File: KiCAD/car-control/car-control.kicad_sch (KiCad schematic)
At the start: 25 parts, among them J1 USB_B_Micro, J2 Conn_01x06, J3 USB_A, J4 Conn_01x04, SW1 SW_Push, SW2 SW_Push, SW3 SW_Push, SW4 SW_Push, SW5 COM-15140, U1 OLED-SSD1322

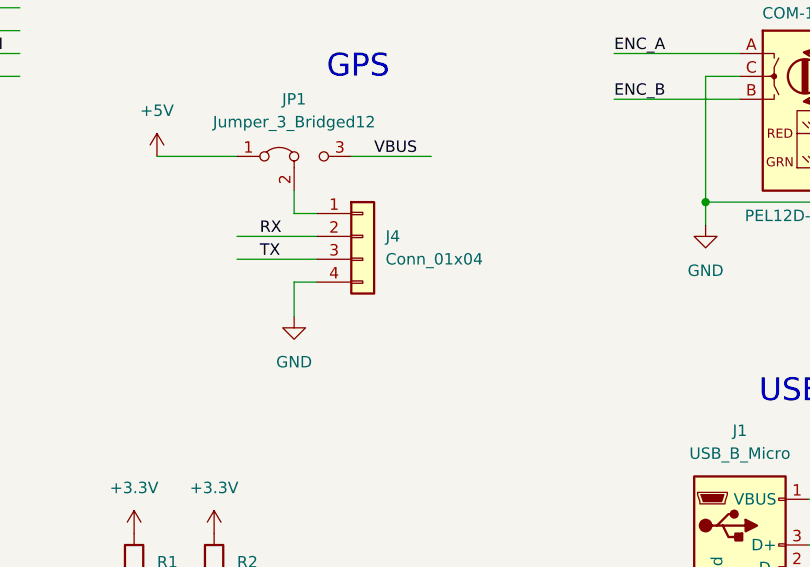
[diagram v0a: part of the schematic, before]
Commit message: PCB V1.0 as built
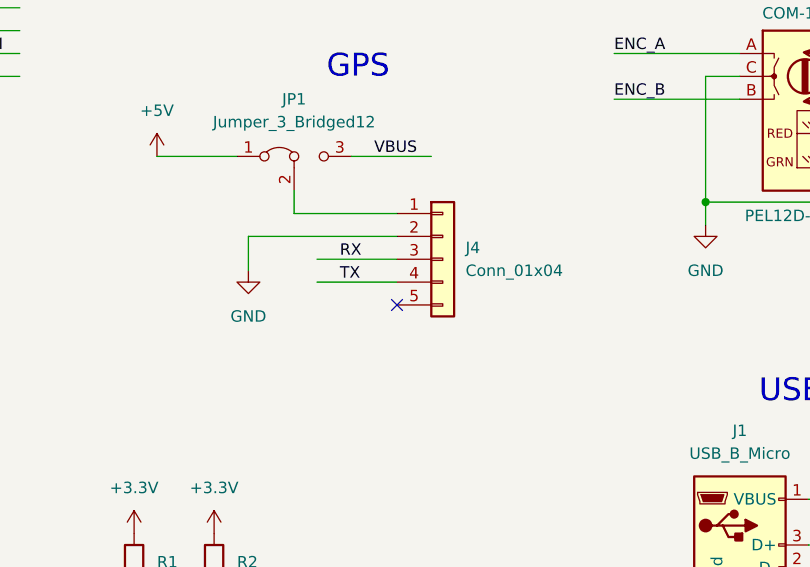
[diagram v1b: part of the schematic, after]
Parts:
- J4: footprint Connector_PinSocket_2.54mm:PinSocket_1x04_P2.54mm_Vertical -> Connector_PinSocket_2.54mm:PinSocket_1x05_P2.54mm_Vertical; symbol Connector_Generic:Conn_01x04 -> Connector_Generic:Conn_01x05
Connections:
- net GND: now also J4.2 (Pin_2); no longer J4.4 (Pin_4)
- net RX: now also J4.3 (Pin_3); no longer J4.2 (Pin_2)
- net TX: now also J4.4 (Pin_4); no longer J4.3 (Pin_3)
- no-connect marks 2 -> 3
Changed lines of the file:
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@@
+	)
+	(no_connect
+		(at 134.62 116.84)
 	)
 	(no_connect
@@
 	(wire
 		(pts
-			(xy 116.84 109.22) (xy 125.73 109.22)
+			(xy 125.73 111.76) (xy 134.62 111.76)
 		)
 		(stroke
@@
 	(wire
 		(pts
-			(xy 125.73 106.68) (xy 123.19 106.68)
+			(xy 123.19 106.68) (xy 134.62 106.68)
 		)
 		(stroke
@@
 	(wire
 		(pts
-			(xy 116.84 111.76) (xy 125.73 111.76)
+			(xy 125.73 114.3) (xy 134.62 114.3)
 		)
 		(stroke
@@
 	(wire
 		(pts
-			(xy 123.19 114.3) (xy 123.19 118.11)
+			(xy 118.11 109.22) (xy 118.11 113.03)
 		)
 		(stroke
@@
 	(wire
 		(pts
-			(xy 125.73 114.3) (xy 123.19 114.3)
+			(xy 118.11 109.22) (xy 134.62 109.22)
 		)
 		(stroke
@@
 	)
 	(label "RX"
-		(at 119.38 109.22 0)
+		(at 128.27 111.76 0)
 		(effects
 			(font
@@
 	)
 	(label "TX"
-		(at 119.38 111.76 0)
+		(at 128.27 114.3 0)
 		(effects
 			(font
@@
 	(symbol
 		(lib_id "power:GND")
-		(at 123.19 118.11 0)
+		(at 118.11 113.03 0)
 		(unit 1)
 		(exclude_from_sim no)
@@
 		(fields_autoplaced yes)
 		(property "Reference" "#PWR014"
-			(at 123.19 124.46 0)
+			(at 118.11 119.38 0)
 			(effects
 				(font
@@
 		)
 		(property "Value" "GND"
-			(at 123.19 123.19 0)
+			(at 118.11 118.11 0)
 			(effects
 				(font
@@
 		)
 		(property "Footprint" ""
-			(at 123.19 118.11 0)
+			(at 118.11 113.03 0)
 			(effects
 				(font
@@
 		)
 		(property "Datasheet" ""
-			(at 123.19 118.11 0)
+			(at 118.11 113.03 0)
 			(effects
 				(font
@@
 		)
 		(property "Description" ""
-			(at 123.19 118.11 0)
+			(at 118.11 113.03 0)
 			(effects
 				(font
@@
 	)
 	(symbol
-		(lib_id "Connector_Generic:Conn_01x04")
-		(at 130.81 109.22 0)
+		(lib_id "Connector_Generic:Conn_01x05")
+		(at 139.7 111.76 0)
 		(unit 1)
 		(exclude_from_sim no)
@@
 		(fields_autoplaced yes)
 		(property "Reference" "J4"
-			(at 133.35 109.2199 0)
+			(at 142.24 110.4899 0)
 			(effects
 				(font
@@
 		)
 		(property "Value" "Conn_01x04"
-			(at 133.35 111.7599 0)
+			(at 142.24 113.0299 0)
 			(effects
 				(font
@@
 			)
 		)
-		(property "Footprint" "Connector_PinSocket_2.54mm:PinSocket_1x04_P2.54mm_Vertical"
-			(at 130.81 109.22 0)
+		(property "Footprint" "Connector_PinSocket_2.54mm:PinSocket_1x05_P2.54mm_Vertical"
+			(at 139.7 111.76 0)
 			(effects
 				(font
@@
 		)
 		(property "Datasheet" "~"
-			(at 130.81 109.22 0)
-			(effects
-				(font
-					(size 1.27 1.27)
-				)
-				(hide yes)
-			)
-		)
-		(property "Description" "Generic connector, single row, 01x04, script generated (kicad-library-utils/schlib/autogen/connector/)"
-			(at 130.81 109.22 0)
+			(at 139.7 111.76 0)
+			(effects
+				(font
+					(size 1.27 1.27)
+				)
+				(hide yes)
+			)
+		)
+		(property "Description" "Generic connector, single row, 01x05, script generated (kicad-library-utils/schlib/autogen/connector/)"
+			(at 139.7 111.76 0)
 			(effects
 				(font
@@
 		(pin "3"
 		)
+		(pin "5"
+		)
 		(instances
